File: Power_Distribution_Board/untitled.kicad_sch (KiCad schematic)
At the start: 50 parts, among them J1 XT60PW-F, J10 XT60PW-F, J11 XT60PW-F, J12 XT60PW-F, J13 XT60PW-F, J14 XT60PW-F, J15 XT30PW-F, J16 XT30PW-F, J17 XT30PW-F, J18 XT30PW-F, J19 XT30PW-F, J2 XT60PW-F, J20 XT30PW-F, J21 XT60PW-F, J22 XT60PW-F, J23 XT60PW-F, J24 XT60PW-F, J25 XT60PW-F, J26 XT60PW-F, J27 XT60PW-F, J3 XT60PW-F, J4 XT60PW-F, J5 DCM3623T75H26C2T00, J6 XT60PW-F, J7 XT60PW-F, J8 XT60PW-F, J9 XT60PW-F

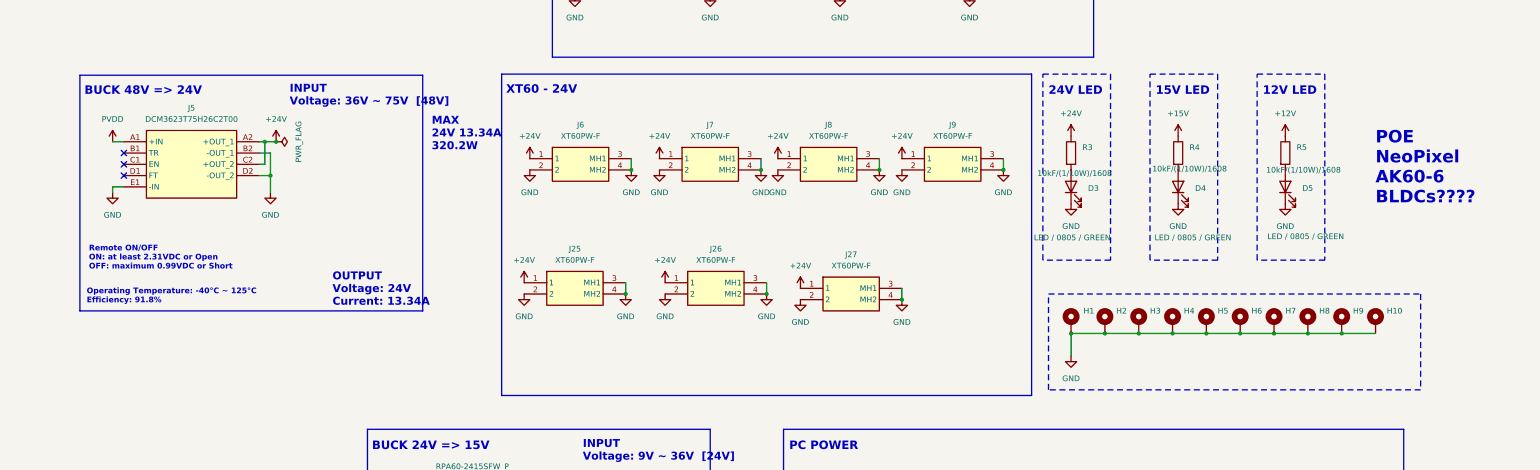
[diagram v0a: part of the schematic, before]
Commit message: Buck changed
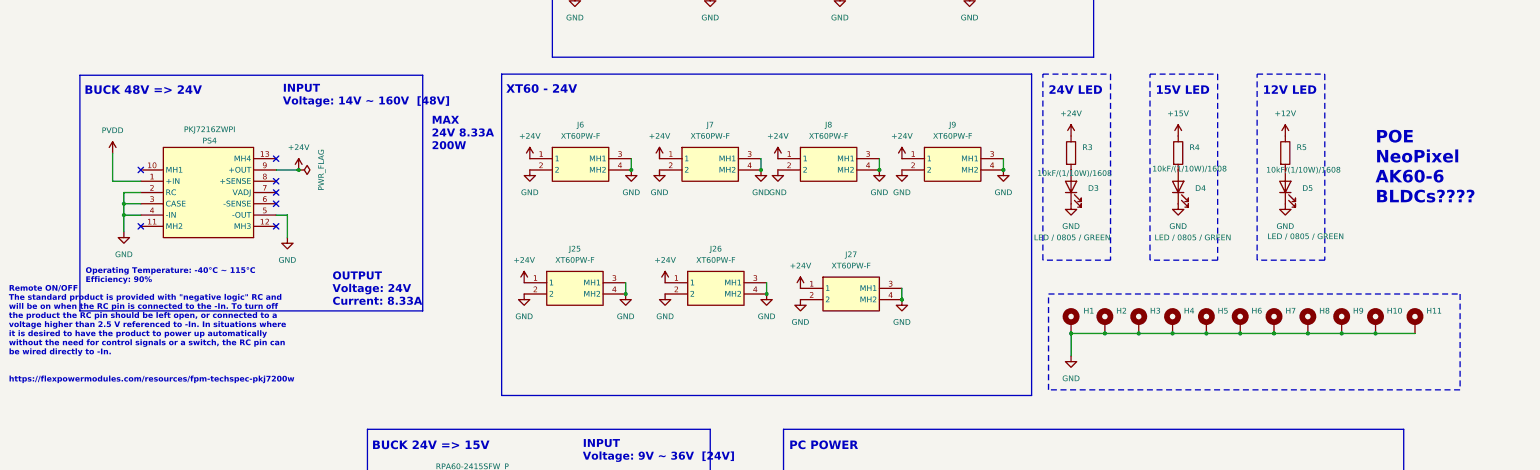
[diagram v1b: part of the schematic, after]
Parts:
- removed J5: DCM3623T75H26C2T00, URC_Active:DCM3623T75H26C2T00, symbol URC_Converter:DCM3623T75H26C2T00
- added H11: MountingHole_Pad, MountingHole:MountingHole_3.2mm_M3_Pad, symbol Mechanical:MountingHole_Pad
- added PS4: PKJ7216ZWPI, PKJ7216ZWPI, symbol URC_Converter:PKJ7216ZWPI
- J1, J10, J11, J12, J13, J14, J2, J21, J22, J23, J24, J25, J26, J27, J3, J4, J6, J7, J8, J9: footprint URC_Con:XT60PWF -> URC_Conn:XT60PWF
- J15, J16, J17, J18, J19, J20: footprint URC_Con:XT30PWF -> URC_Conn:XT30PWF
- PS1: footprint URC_Con:XT60PWM -> URC_Conn:XT60PWM
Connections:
- net +24V: now also PS4.9 (+OUT)
- net GND: now also H11.1, PS4.2 (RC), PS4.3 (CASE), PS4.4 (-IN), PS4.5 (-OUT)
- net PVDD: now also PS4.1 (+IN)
- no-connect marks 9 -> 13
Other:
- note added: "INPUT Voltage: 14V ~ 160V [48V]"
- note added: "MAX 24V 8.33A 200W"
- note added: "OUTPUT Voltage: 24V Current: 8.33A"
- note added: "Operating Temperature: -40°C ~ 115°C Efficiency: 90%"
- note added: "Remote ON/OFF The standard product is provided with "negative logic" RC and will be on when the RC pin is connected to the -In. To turn off the product the RC pin should be left open, or connected to a voltage higher than 2.5 V referenced to -In. In situations where it is desired to have the product to power up automatically without the need for control signals or a switch, the RC pin can be wire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"
- note removed: "INPUT Voltage: 36V ~ 75V [48V]"
- note removed: "MAX 24V 13.34A 320.2W"
- note removed: "OUTPUT Voltage: 24V Current: 13.34A"
- note removed: "Operating Temperature: -40°C ~ 125°C Efficiency: 91.8%"
- note removed: "Remote ON/OFF ON: at least 2.31VDC or Open OFF: maximum 0.99VDC or Short"
